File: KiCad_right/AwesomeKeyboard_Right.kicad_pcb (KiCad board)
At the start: 2 copper layers, 140 x 109 mm, 54 parts, among them J1 AudioJack4_Ground, SW1 SW_DIP_x01, SW11 SW_Push, SW12 SW_Push, SW13 SW_Push, SW14 SW_Push, SW15 SW_Push, SW16 SW_Push, SW21 SW_Push, SW22 SW_Push, SW23 SW_Push, SW24 SW_Push, SW25 SW_Push, SW26 SW_Push, SW31 SW_Push, SW32 SW_Push, SW33 SW_Push, SW34 SW_Push, SW35 SW_Push, SW36 SW_Push, SW45 SW_Push, SW46 SW_Push

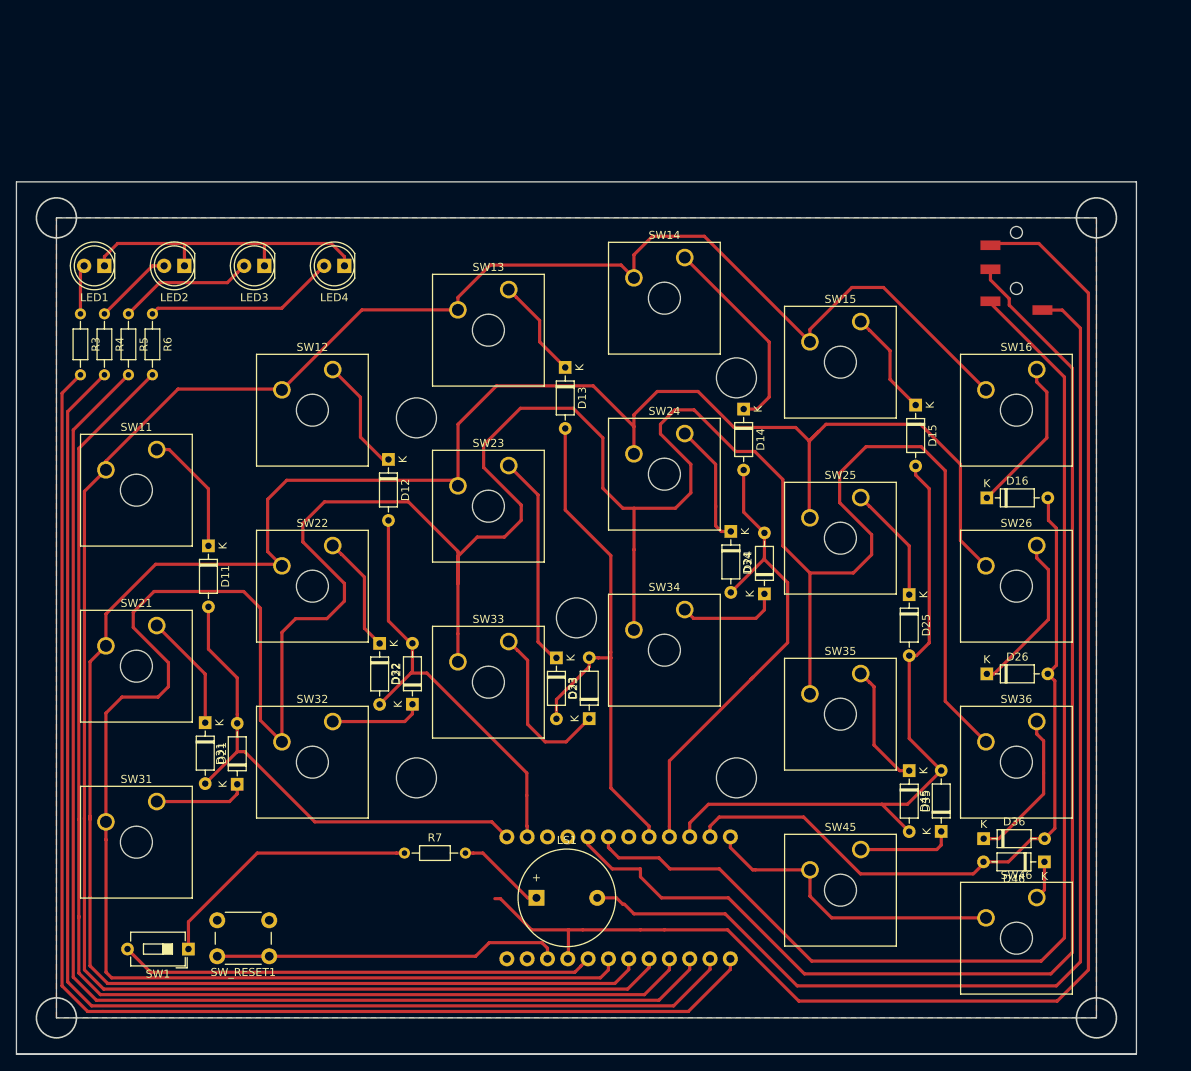
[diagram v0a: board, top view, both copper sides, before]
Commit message: right
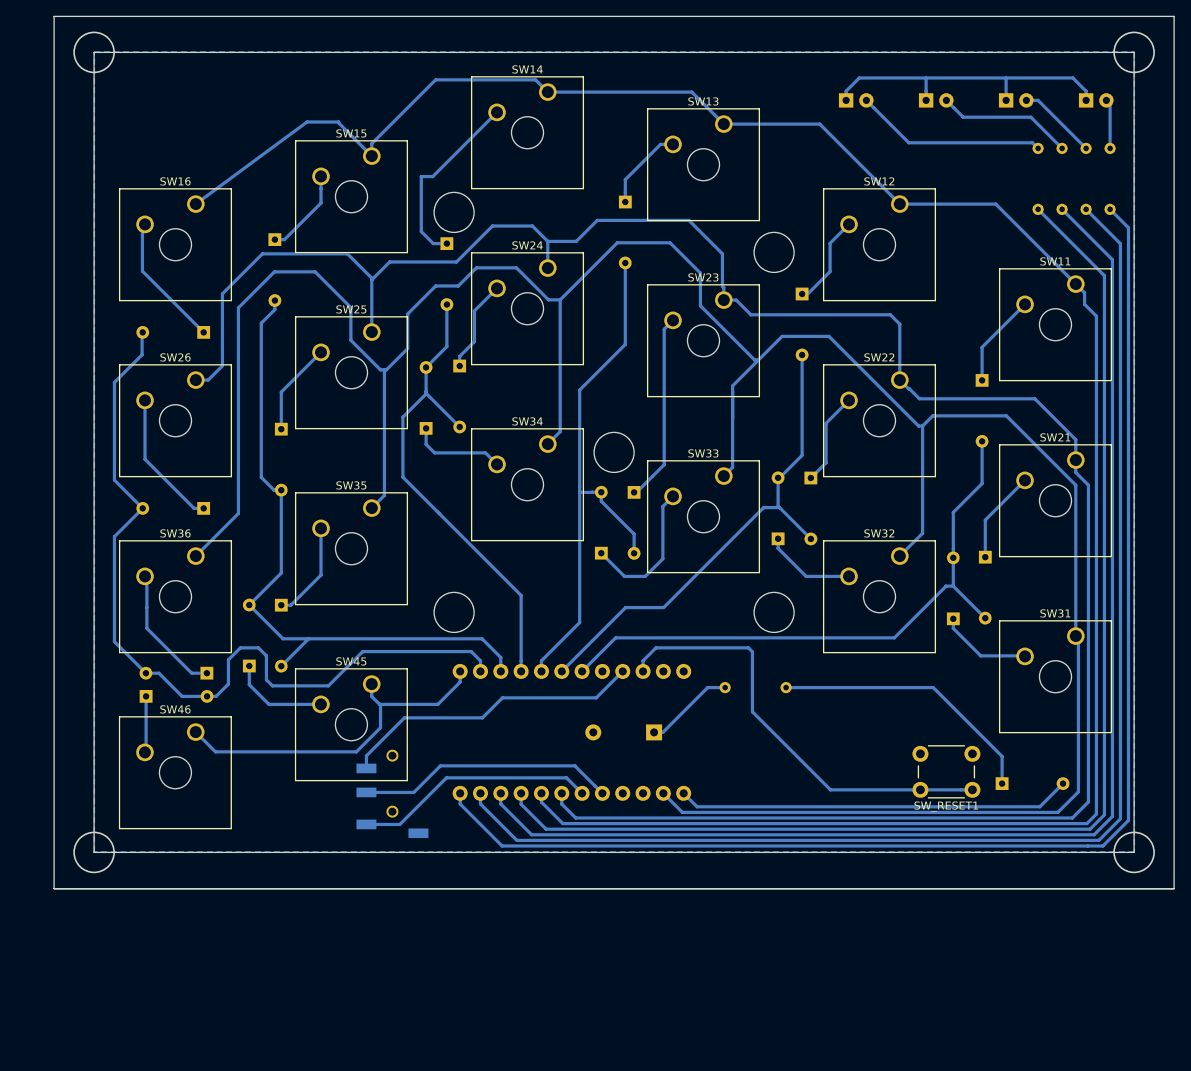
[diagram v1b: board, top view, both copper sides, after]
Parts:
- D11, D12, D13, D14, D15, D16, D21, D22, D23, D24, D25, D26, D31, D32, D33, D34, D35, D36, D45, D46, LED1, LED2, LED3, LED4, LS1, R3, R4, R5, R6, R7, SW1: moved to B.Cu
- moved R3 130.4 mm to (209.5, 66.0)
- moved LED1 124.4 mm to (206.5, 60.0), turned to 0 degrees
- moved R4 124.4 mm to (206.5, 66.0)
- moved R5 118.5 mm to (203.5, 66.0)
- moved SW11 116.7 mm to (205.2, 82.9)
- moved SW21 116.7 mm to (205.2, 104.9)
- moved SW31 116.7 mm to (205.2, 126.9)
- moved D46 114.2 mm to (89.0, 134.5), turned to 0 degrees
- moved R6 112.6 mm to (200.5, 66.0)
- moved SW46 107.1 mm to (95.2, 138.9)
- moved SW16 107.1 mm to (95.2, 72.9)
- moved SW26 107.1 mm to (95.2, 94.9)
- moved SW36 107.1 mm to (95.2, 116.9)
- moved LED2 104.8 mm to (196.5, 60.0), turned to 0 degrees
- moved SW1 103.8 mm to (196.0, 145.4), turned to 0 degrees
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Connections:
- B1 pad 1: /COL1 -> /SPEAKER
- B1 pad 10: /COL5 -> /LED3
- B1 pad 11: /COL6 -> /LED2
- B1 pad 12: /ROW4 -> /LED1
- B1 pad 13: /LED1 -> /ROW4
- B1 pad 14: /LED2 -> /COL6
- B1 pad 15: /LED3 -> /COL5
- B1 pad 16: /LED4 -> /COL4
- B1 pad 17: /ROW1 -> /COL3
- B1 pad 18: /ROW2 -> /COL2
- B1 pad 19: /ROW3 -> /COL1
- B1 pad 2: /COL2 -> /ROW3
- B1 pad 20: /SPEAKER -> (no net)
- B1 pad 21: (no net) -> VCC
- B1 pad 23: (no net) -> GND
- B1 pad 3: (no net) -> GND
- B1 pad 4: (no net) -> GND
- B1 pad 7: (no net) -> /ROW2
- B1 pad 8: /COL3 -> /ROW1
- B1 pad 9: /COL4 -> /LED4
- J1 pad 3: (no net) -> VCC
- SW11 pad 1: Net-(D11-Pad1) -> /ROW1
- SW11 pad 2: /ROW1 -> Net-(D11-Pad1)
- SW12 pad 1: Net-(D12-Pad1) -> /ROW1
- SW12 pad 2: /ROW1 -> Net-(D12-Pad1)
- SW13 pad 1: Net-(D13-Pad1) -> /ROW1
- SW13 pad 2: /ROW1 -> Net-(D13-Pad1)
- SW14 pad 1: Net-(D14-Pad1) -> /ROW1
- SW14 pad 2: /ROW1 -> Net-(D14-Pad1)
- SW15 pad 1: Net-(D15-Pad1) -> /ROW1
- SW15 pad 2: /ROW1 -> Net-(D15-Pad1)
- SW16 pad 1: Net-(D16-Pad1) -> /ROW1
- SW16 pad 2: /ROW1 -> Net-(D16-Pad1)
- SW21 pad 1: Net-(D21-Pad1) -> /ROW2
- SW21 pad 2: /ROW2 -> Net-(D21-Pad1)
- SW22 pad 1: Net-(D22-Pad1) -> /ROW2
- SW22 pad 2: /ROW2 -> Net-(D22-Pad1)
- SW23 pad 1: Net-(D23-Pad1) -> /ROW2
- SW23 pad 2: /ROW2 -> Net-(D23-Pad1)
- SW24 pad 1: Net-(D24-Pad1) -> /ROW2
- SW24 pad 2: /ROW2 -> Net-(D24-Pad1)
- SW25 pad 1: Net-(D25-Pad1) -> /ROW2
- SW25 pad 2: /ROW2 -> Net-(D25-Pad1)
- SW26 pad 1: Net-(D26-Pad1) -> /ROW2
- SW26 pad 2: /ROW2 -> Net-(D26-Pad1)
- SW31 pad 1: Net-(D31-Pad1) -> /ROW3
- SW31 pad 2: /ROW3 -> Net-(D31-Pad1)
- SW32 pad 1: Net-(D32-Pad1) -> /ROW3
- SW32 pad 2: /ROW3 -> Net-(D32-Pad1)
- SW33 pad 1: Net-(D33-Pad1) -> /ROW3
- SW33 pad 2: /ROW3 -> Net-(D33-Pad1)
- SW34 pad 1: Net-(D34-Pad1) -> /ROW3
- SW34 pad 2: /ROW3 -> Net-(D34-Pad1)
- SW35 pad 1: Net-(D35-Pad1) -> /ROW3
- SW35 pad 2: /ROW3 -> Net-(D35-Pad1)
- SW36 pad 1: Net-(D36-Pad1) -> /ROW3
- SW36 pad 2: /ROW3 -> Net-(D36-Pad1)
- SW45 pad 1: Net-(D45-Pad1) -> /ROW4
- SW45 pad 2: /ROW4 -> Net-(D45-Pad1)
- SW46 pad 1: Net-(D46-Pad1) -> /ROW4
- SW46 pad 2: /ROW4 -> Net-(D46-Pad1)
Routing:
- net (no net): track 184.3 -> 0.00 mm
- net GND: track 190.4 -> 39.3 mm
- net Net-(B1-Pad5): track 159.5 -> 32.3 mm
- net Net-(B1-Pad6): track 148.8 -> 30.2 mm
- net /ROW3: track 432.7 -> 344.2 mm
- net VCC: track 0.00 -> 38.1 mm
- net /ROW2: track 285.7 -> 271.2 mm
- net /COL1: track 63.4 -> 76.1 mm
- net Net-(B1-Pad22): track 43.6 -> 54.9 mm
- net /COL6: track 92.6 -> 103.2 mm
- net /SPEAKER: track 59.5 -> 49.3 mm
- net /ROW1: track 278.8 -> 270.0 mm
- net /COL2: track 53.8 -> 61.8 mm
- net /ROW4: track 38.9 -> 43.8 mm
- net Net-(D24-Pad1): track 15.5 -> 11.6 mm
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- added copper zone on B.Cu, net GND
- removed copper zone on F.Cu, net GND
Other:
- outline, holes or cut-outs redrawn

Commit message: right
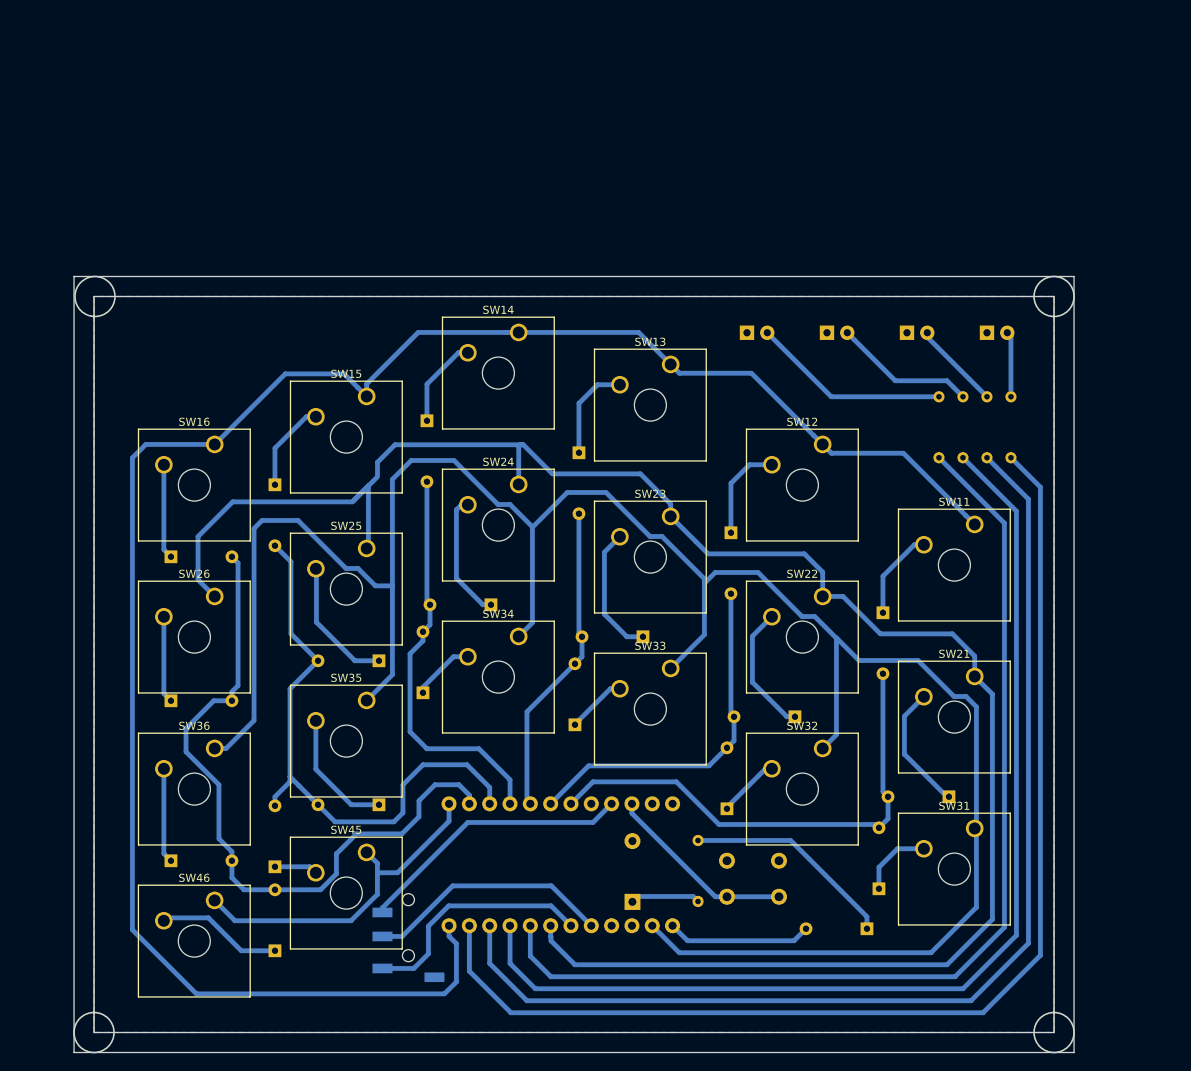
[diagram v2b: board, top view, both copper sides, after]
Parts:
- SW_RESET1: moved to B.Cu
- moved D46 35.6 mm to (105.1, 166.3), turned to 90 degrees
- moved D31 35.0 mm to (180.6, 158.5)
- moved D32 34.3 mm to (161.6, 148.5)
- moved SW_RESET1 33.5 mm to (161.6, 159.5), turned to 0 degrees
- moved R3 33.4 mm to (197.1, 97.0)
- moved R4 33.4 mm to (194.1, 97.0)
- moved R5 33.4 mm to (191.1, 97.0)
- moved R6 33.4 mm to (188.1, 97.0)
- moved D34 33.0 mm to (123.6, 134.0)
- moved SW11 32.6 mm to (192.6, 113.0)
- moved D13 31.9 mm to (143.1, 104.0)
- moved LED1 31.6 mm to (194.1, 89.0)
- moved LED2 31.6 mm to (184.1, 89.0)
- moved LED3 31.6 mm to (174.1, 89.0)
- moved LED4 31.6 mm to (164.1, 89.0)
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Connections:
- B1 pad 10: /LED3 -> /LED2
- B1 pad 11: /LED2 -> /LED1
- B1 pad 12: /LED1 -> /ROW1
- B1 pad 8: /ROW1 -> /LED4
- B1 pad 9: /LED4 -> /LED3
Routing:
- net /ROW3: track 344.2 -> 283.0 mm
- net GND: track 39.3 -> 0.00 mm
- net /ROW2: track 271.2 -> 234.8 mm
- net /ROW1: track 270.0 -> 235.8 mm
- net /SPEAKER: track 49.3 -> 18.1 mm
- net Net-(B1-Pad22): track 54.9 -> 23.9 mm
- net /COL3: track 67.7 -> 39.4 mm
- net /LED4: track 155.4 -> 128.8 mm
- net /LED3: track 158.8 -> 134.6 mm
- net /LED2: track 162.3 -> 139.8 mm
- net /LED1: track 165.7 -> 145.9 mm
- net /COL2: track 61.8 -> 44.7 mm
- net /COL6: track 103.2 -> 87.0 mm
- net /COL1: track 76.1 -> 62.0 mm
- net Net-(D14-Pad1): track 23.5 -> 11.3 mm
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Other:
- board size 140 x 109 mm -> 125 x 97 mm
- net class Default: trace_width 0.4 -> 0.6
